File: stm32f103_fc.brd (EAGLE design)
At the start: 53.1 x 76.5 mm, 50 parts, among them IC1 STM32F103C8T6, IC2 LD1117AS33TR, Y1 8MHz, Y2 32.768MHz

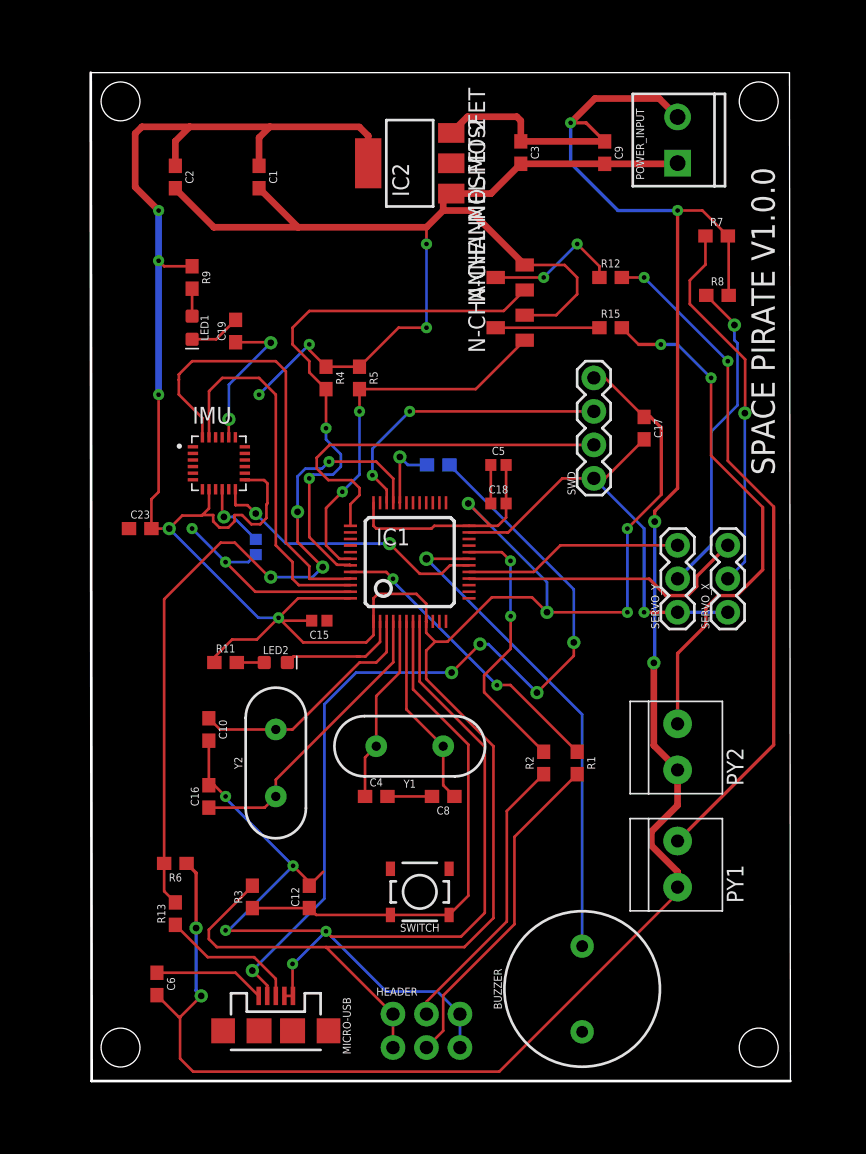
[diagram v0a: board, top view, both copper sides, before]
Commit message: version 1.0.1 done
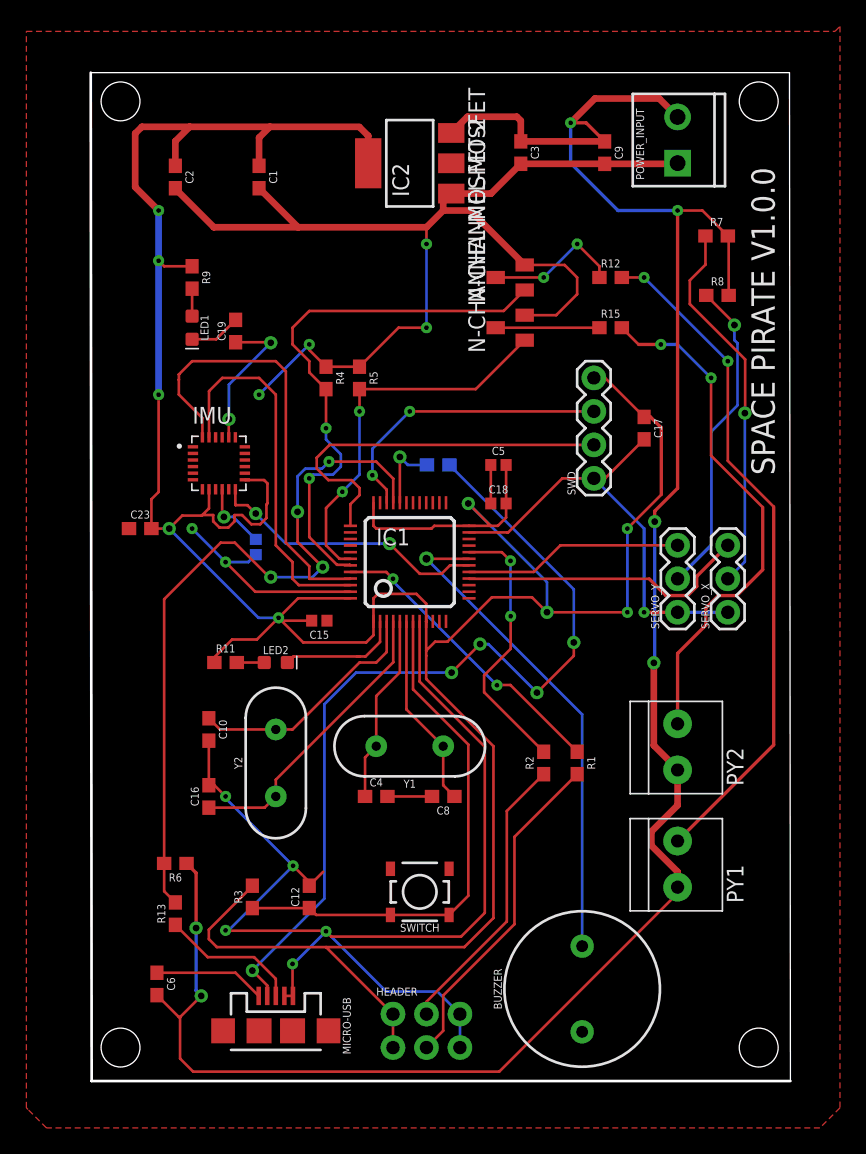
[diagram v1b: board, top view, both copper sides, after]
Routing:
- added copper zone on layer 1, net GND
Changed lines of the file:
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@@
 <wire x1="40.03" y1="83.13419375" x2="40.03" y2="81.0538625" width="0.508" layer="1"/>
 <wire x1="44.43" y1="46.28298125" x2="44.43" y2="46.2802625" width="0.2032" layer="1"/>
-<wire x1="44.43" y1="44.0838125" x2="44.43" y2="41.93" width="0.2032" layer="1"/>
+<wire x1="44.43" y1="44.0838125" x2="44.43" y2="43.688" width="0.2032" layer="1"/>
+<wire x1="44.43" y1="43.688" x2="44.43" y2="41.93" width="0.2032" layer="1"/>
 <wire x1="44.43" y1="41.93" x2="49.53" y2="36.83" width="0.2032" layer="1"/>
 <wire x1="44.43" y1="46.28298125" x2="44.43298125" y2="46.28" width="0.2032" layer="1"/>
@@
 <wire x1="35.742" y1="46.355" x2="33.4474" y2="46.355" width="0.2032" layer="1"/>
 <wire x1="33.4474" y1="46.355" x2="33.23" y2="46.5724" width="0.2032" layer="1"/>
-<wire x1="41.91" y1="13.97" x2="41.91" y2="13.716" width="0.2032" layer="1"/>
 <wire x1="40.43" y1="55.3" x2="40.43" y2="53.55" width="0.2032" layer="1"/>
 <wire x1="40.43" y1="53.55" x2="40.64" y2="53.34" width="0.2032" layer="1"/>
@@
 <wire x1="40.43" y1="48.05" x2="40.767" y2="48.387" width="0.2032" layer="1"/>
 <wire x1="40.767" y1="48.387" x2="43.688" y2="48.387" width="0.2032" layer="1"/>
-<wire x1="43.688" y1="48.387" x2="44.43" y2="47.645" width="0.2032" layer="1"/>
+<wire x1="44.43" y1="47.645" x2="43.688" y2="48.387" width="0.2032" layer="1"/>
 <wire x1="44.43" y1="46.3" x2="44.4302625" y2="46.2997375" width="0.2032" layer="1"/>
 <wire x1="44.4302625" y1="46.2997375" x2="44.4302625" y2="46.28" width="0.2032" layer="1"/>
-<wire x1="44.43" y1="46.3" x2="44.43" y2="45.43646875" width="0.2032" layer="1"/>
-<wire x1="44.43" y1="45.43646875" x2="45.106328125" y2="44.760140625" width="0.2032" layer="1"/>
-<wire x1="44.43" y1="47.645" x2="44.43" y2="46.3" width="0.2032" layer="1"/>
+<wire x1="44.43" y1="46.3" x2="44.43" y2="47.645" width="0.2032" layer="1"/>
+<wire x1="44.43" y1="46.3" x2="44.43" y2="44.0838125" width="0.2032" layer="1"/>
 </signal>
 <signal name="N$1">
@@
 <wire x1="28.499" y1="67.703" x2="29.972" y2="69.176" width="0.2032" layer="1"/>
 <wire x1="28.321" y1="76.2" x2="34.71" y2="76.2" width="0.508" layer="1"/>
-<wire x1="50.60064375" y1="53.05" x2="49.331" y2="55.245" width="0" layer="19" extent="1-1"/>
-<wire x1="40.93" y1="55.3" x2="47.68" y2="53.05" width="0" layer="19" extent="1-1"/>
-<wire x1="38.68" y1="48.55" x2="40.93" y2="55.3" width="0" layer="19" extent="1-1"/>
-<wire x1="36.902" y1="46.355" x2="38.68" y2="48.55" width="0" layer="19" extent="1-1"/>
-<wire x1="29.452" y1="56.323" x2="26.67" y2="53.34" width="0" layer="19" extent="1-1"/>
-<wire x1="30.672" y1="59.543" x2="29.452" y2="56.323" width="0" layer="19" extent="1-1"/>
-<wire x1="26.732" y1="59.543" x2="30.672" y2="59.543" width="0" layer="19" extent="1-1"/>
-<wire x1="31.75" y1="63.5" x2="30.672" y2="59.543" width="0" layer="19" extent="1-1"/>
-<wire x1="21.883" y1="53.34" x2="26.67" y2="53.34" width="0" layer="19" extent="1-1"/>
-<wire x1="28.499" y1="67.703" x2="31.75" y2="63.5" width="0" layer="19" extent="1-1"/>
-<wire x1="43.93" y1="46.3" x2="38.68" y2="48.55" width="0" layer="19" extent="1-1"/>
-<wire x1="46.167" y1="27.531" x2="48.87308125" y2="24.1875" width="0" layer="19" extent="1-1"/>
-<wire x1="41.717" y1="27.531" x2="46.167" y2="27.531" width="0" layer="19" extent="1-1"/>
-<wire x1="44.87" y1="33.02" x2="48.87308125" y2="36.791665625" width="0" layer="19" extent="1-1"/>
-<wire x1="56.261" y1="15.165" x2="46.99" y2="13.97" width="0" layer="19" extent="1-1"/>
+<polygon width="0.2032" layer="1">
+<vertex x="14.097" y="91.059"/>
+<vertex x="75.438" y="91.059"/>
+<vertex x="75.819" y="91.44"/>
+<vertex x="75.819" y="9.398"/>
+<vertex x="74.295" y="7.874"/>
+<vertex x="15.621" y="7.874"/>
+<vertex x="14.224" y="9.271"/>
+<vertex x="14.097" y="9.398"/>
+</polygon>
 </signal>
 <signal name="N$3">
@@
 <contactref element="R10" pad="2"/>
 <contactref element="IC1" pad="32"/>
-<wire x1="42.41035" y1="55.31965" x2="42.43" y2="55.3" width="0.2032" layer="1"/>
 <wire x1="42.43" y1="55.3" x2="42.43" y2="58.774" width="0.2032" layer="1"/>
 <wire x1="43.038" y1="58.166" x2="44.489" y2="58.166" width="0.2032" layer="16"/>
